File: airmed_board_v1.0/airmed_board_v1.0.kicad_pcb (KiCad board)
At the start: 2 copper layers, 76.4 x 49.6 mm, 61 parts, among them J1 Barrel_Jack, J2 Conn_02x03_Odd_Even, J3 Conn_02x15_Top_Bottom, J5 Conn_02x05_Odd_Even, SW1 SW_SPDT, SW2 SW_Push, U1 AP1084K50L-13, U2 AZ1084CD-3.3TRG1, U3 CC3220, U4 DEA202450BT-1294C1-H, U5 MX25R3235F, Y1 Crystal_GND24, Y2 Crystal

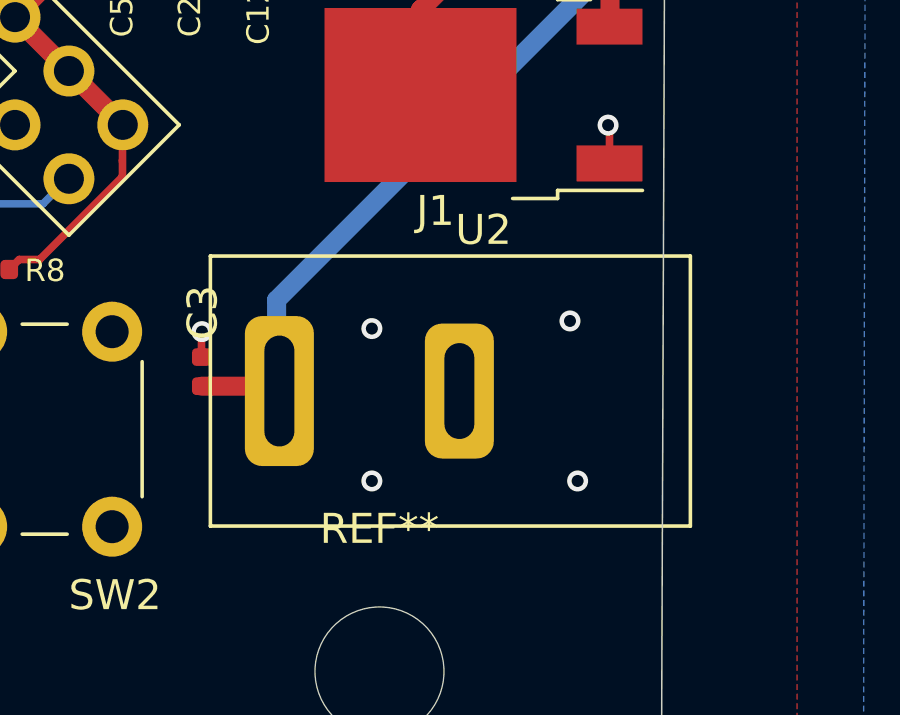
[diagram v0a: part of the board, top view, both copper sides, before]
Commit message: added so many things
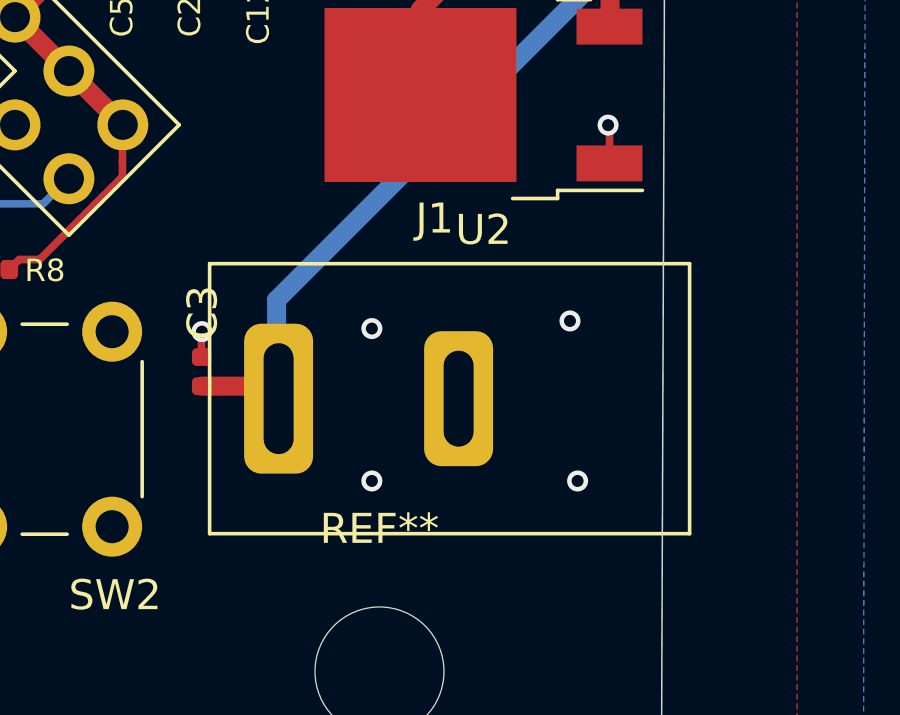
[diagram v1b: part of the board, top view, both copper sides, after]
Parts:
- moved J1 0.26 mm to (180.6, 104.8)
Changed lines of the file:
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@@
       (padsonsilk false)
       (subtractmaskfromsilk false)
-      (outputformat 1)
+      (outputformat 4)
       (mirror false)
       (drillshape 0)
       (scaleselection 1)
-      (outputdirectory "gerbers/"))
+      (outputdirectory "../../../../../../../../../Desktop/"))
   )
   (net 0 "")
@@
   )
   (module Connector_BarrelJack:BarrelJack_CUI_PJ-037A_Horizontal (layer F.Cu)
-    (at 180.6232 104.5328 180)
+    (at 180.5978 104.7868 180)
     (fp_text reference J1 (at 8.5 6 180) (layer F.SilkS)
       (effects (font (size 1 1) (thickness 0.15)))
@@
   (via (at 148.137736 90.817936) (size 0.6) (drill 0.4) (layers F.Cu B.Cu) (net 1))
   (segment (start 139.5387 101.053) (end 139.0615 100.2284) (width 0.254) (layer F.Cu) (net 1))
-  (via (at 139.5387 101.053) (size 0.508) (drill 0.254) (layers F.Cu B.Cu) (net 1))
+  (via (at 139.5387 101.053) (size 0.508) (drill 0.254) (layers F.Cu B.Cu) (net 1) (status 1000000))
   (segment (start 148.239214 99.630553) (end 148.5303 99.630553) (width 0.254) (layer F.Cu) (net 2))
   (segment (start 146.596245 97.987584) (end 147.997961 99.3893) (width 0.254) (layer F.Cu) (net 2))
